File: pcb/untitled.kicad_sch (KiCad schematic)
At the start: 27 parts, among them U10 LTV-817S, U11 LTV-817S, U3 LTV-817S, U4 LTV-817S, U5 LTV-817S, U6 LTV-817S, U7 LTV-817S, U8 LTV-817S, U9 LTV-817S

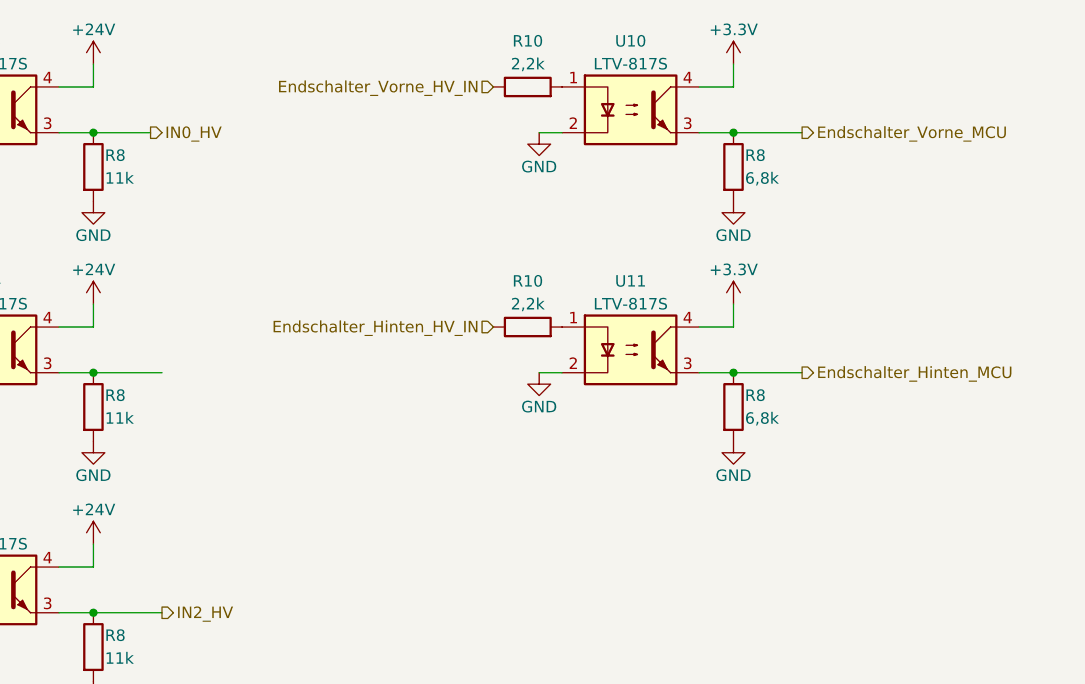
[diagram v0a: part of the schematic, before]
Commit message: updated pcb
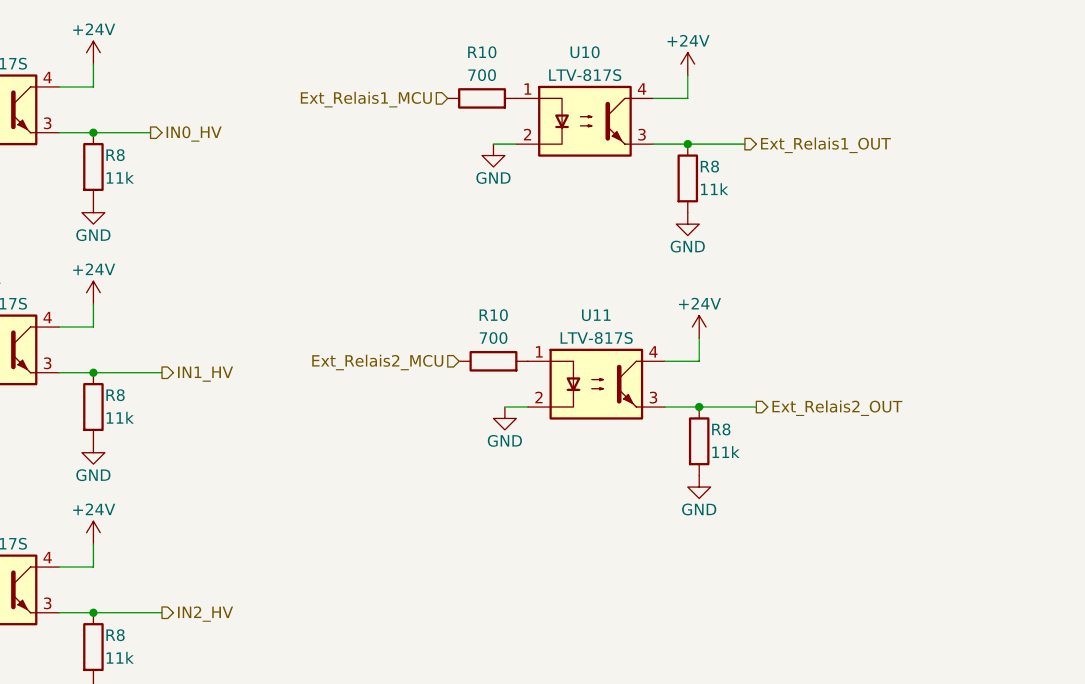
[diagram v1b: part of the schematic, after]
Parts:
- removed R10 (x2): 2,2k, Resistor_SMD:R_1206_3216Metric, symbol Device:R
- removed R8 (x2): 6,8k, Resistor_SMD:R_1206_3216Metric, symbol Device:R
- added R10 (x2): 700, Resistor_SMD:R_1206_3216Metric, symbol Device:R
- added R8 (x2): 11k, Resistor_SMD:R_1206_3216Metric, symbol Device:R
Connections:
- net +24V: now also U10.4, U11.4
- net +3.3V: no longer U10.4, U11.4
- net GND: now also R8.2, R8.2
- net at U11.1: now also R10.2
- net IN1_HV: now reaches R8.1, U4.3
- net at U10.1: now also R10.2
- net Endschalter_Hinten_MCU renamed Ext_Relais2_OUT
- net Ext_Relais2_OUT: now also R8.1
- net Endschalter_Vorne_MCU renamed Ext_Relais1_OUT
- net Ext_Relais1_OUT: now also R8.1
- new net Ext_Relais1_MCU: R10.1
- new net Ext_Relais2_MCU: R10.1
